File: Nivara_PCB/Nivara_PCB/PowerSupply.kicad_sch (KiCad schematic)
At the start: 19 parts, among them U4 AP63200WU

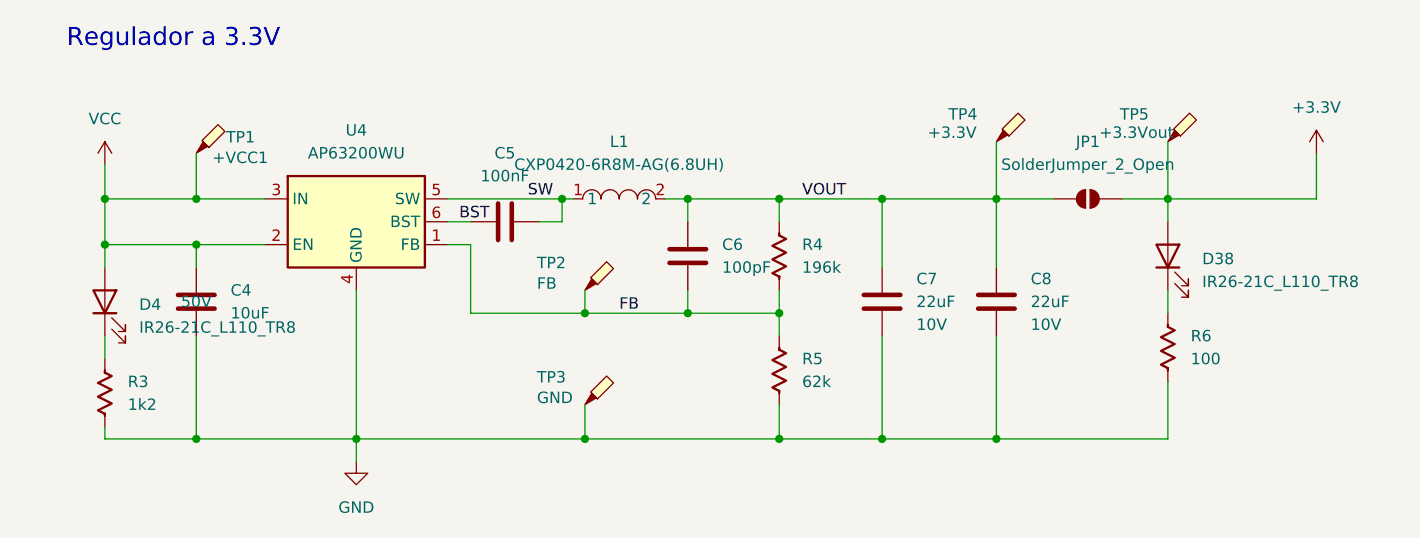
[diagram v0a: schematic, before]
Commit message: TERMINACIONES Y AJUSTES FINALES
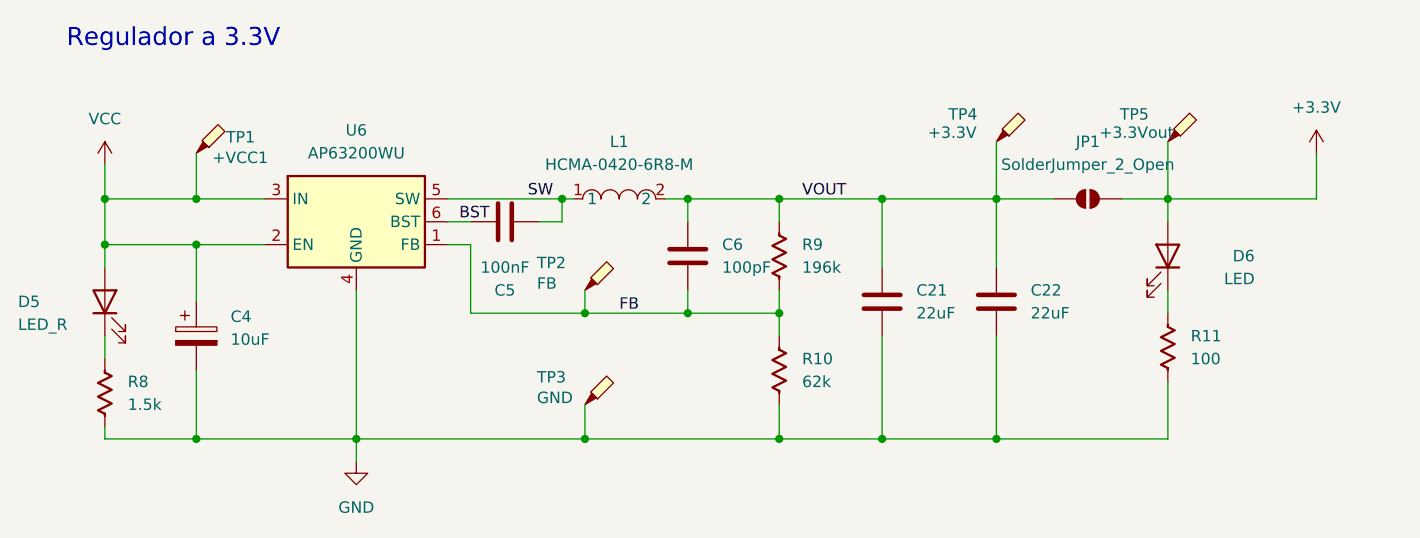
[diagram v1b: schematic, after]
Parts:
- removed C4: 10uF, PCM_Capacitor_SMD_AKL:C_1206_3216Metric, symbol EasyEDA:C_1206
- removed C7, C8: 22uF, PCM_Capacitor_SMD_AKL:C_0603_1608Metric, symbol EasyEDA:C_0603
- removed D38, D4: IR26-21C_L110_TR8, LED_SMD:LED_1206_3216Metric, symbol LED:IR26-21C_L110_TR8
- removed R3: 1k2, PCM_Resistor_SMD_AKL:R_0603_1608Metric, symbol EasyEDA:R_0603
- added C21, C22: 22uF, PCM_Capacitor_SMD_AKL:C_0805_2012Metric, symbol EasyEDA:C_0805
- added C4: 10uF, Capacitor_SMD:CP_Elec_4x5.4, symbol Device:C_Polarized
- added D5: LED_R, LED_SMD:LED_0603_1608Metric, symbol EasyEDA:LED
- added D6: LED, LED_SMD:LED_0603_1608Metric, symbol EasyEDA:LED
- added R8: 1.5k, PCM_Resistor_SMD_AKL:R_0603_1608Metric, symbol EasyEDA:R_0603
- C5: LCSC Part (none) -> C56476; Part # (none) -> C1608X7R1H104KT000N
- C6: LCSC Part (none) -> C76709; Part # (none) -> CGA3E2C0G1H101JT0Y0N
- L1: value CXP0420-6R8M-AG(6.8UH) -> HCMA-0420-6R8-M; LCSC Part C7461340 -> C351092; Part # (none) -> YSPI0420-6R8M
- R10: renamed from R5; LCSC Part (none) -> C136961; Part # (none) -> RT0603BRD0762KL
- R11: renamed from R6; LCSC Part (none) -> C22775; Part # (none) -> 0603WAF1000T5E
- R9: renamed from R4; LCSC Part (none) -> C2974032; Part # (none) -> FRC0603F1963TS
- TP1, TP2, TP3, TP4, TP5: now left out of the parts list
- U6: renamed from U4; LCSC Part (none) -> C2071868; Part # (none) -> AP63200WU-7
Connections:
- net +3.3V: now also D6.2 (A)
- net GND: now also C21.1, C22.1, C4.2, R8.2
- net VCC: now also C4.1, D5.2 (A)
- net VOUT: now also C21.2, C22.2
- net at R11.2: now also D6.1 (K)
- new net: D5.1 (K), R8.1
